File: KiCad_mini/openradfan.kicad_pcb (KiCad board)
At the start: 2 copper layers, 79.5 x 28 mm, 39 parts, among them CN1 DB141V-2.54-3P, J1 Fan_CPU_4pin, J5 Fan_CPU_4pin, Q1 AO3401A_C347476, U1 74AHCT125, U2 AP63205WU, U3 BTS462TATMA1

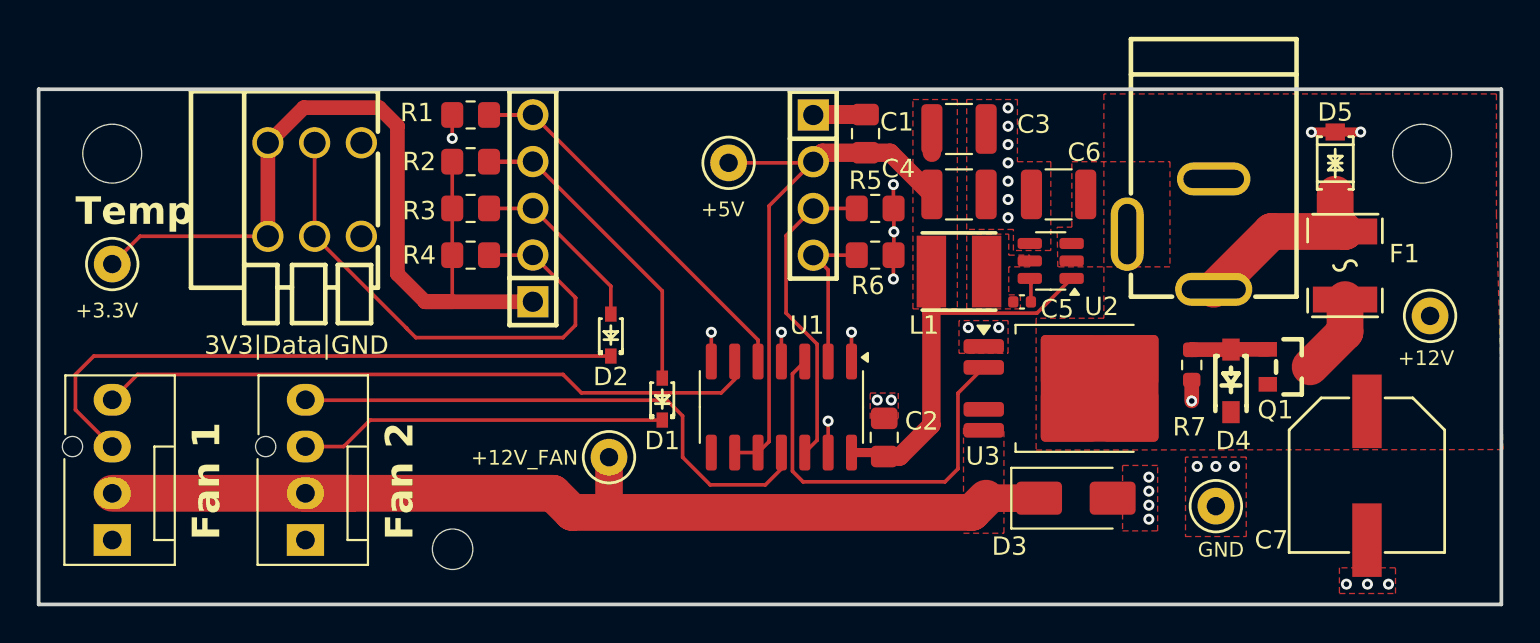
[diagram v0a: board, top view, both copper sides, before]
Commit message: Tweaks
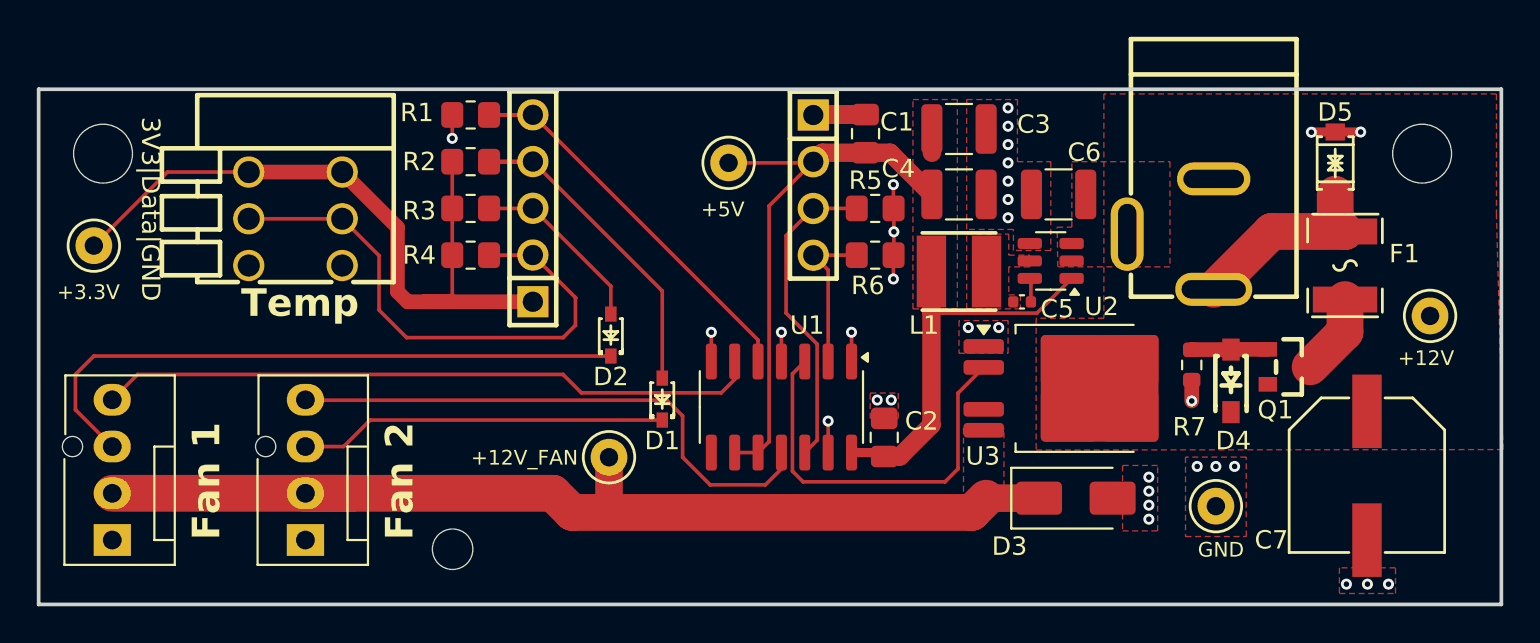
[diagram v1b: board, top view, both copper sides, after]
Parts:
- moved CN1 1.90 mm to (56.5, 68.1), turned to 90 degrees
- moved TP2 1.41 mm to (45.6, 69.6)
- moved H1 0.50 mm to (46.1, 64.6)
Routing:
- net +3.3V: track 48.5 -> 40.6 mm
- net GPIO_DS18B20: track 29.0 -> 29.6 mm
